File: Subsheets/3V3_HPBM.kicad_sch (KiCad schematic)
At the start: 7 parts

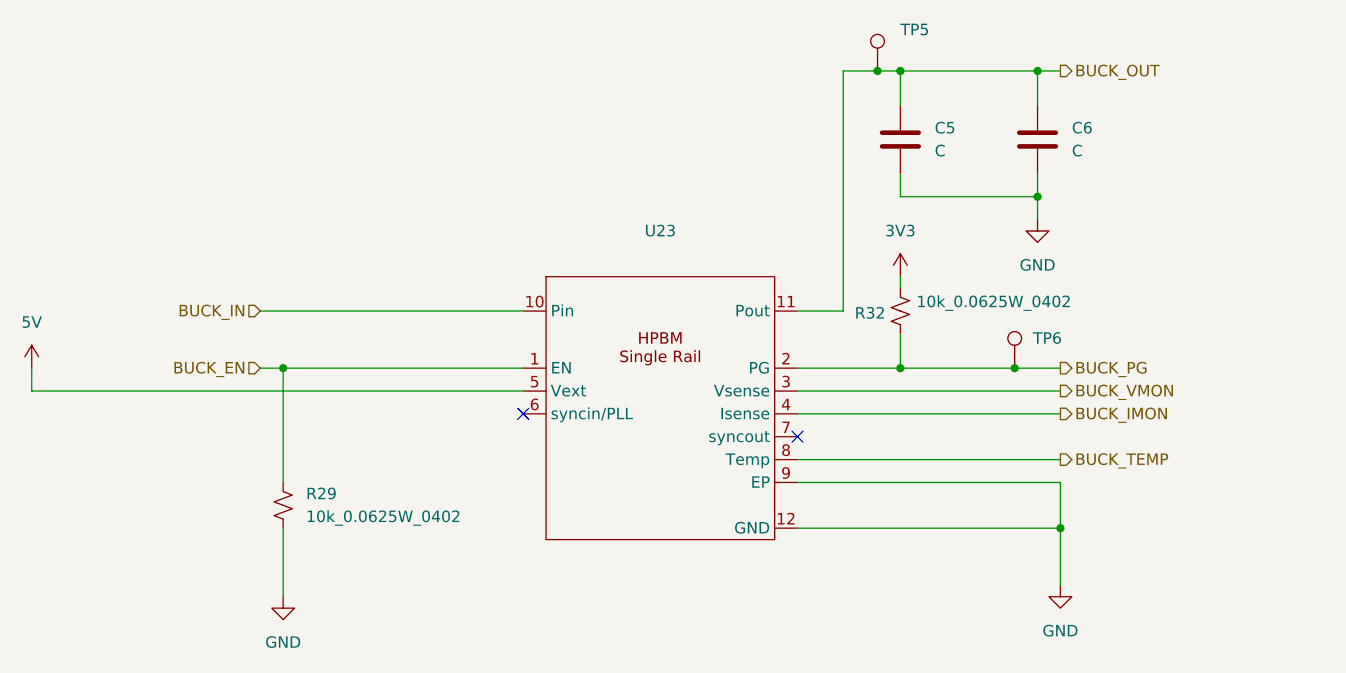
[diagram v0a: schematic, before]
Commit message: Schematic Update-1.1
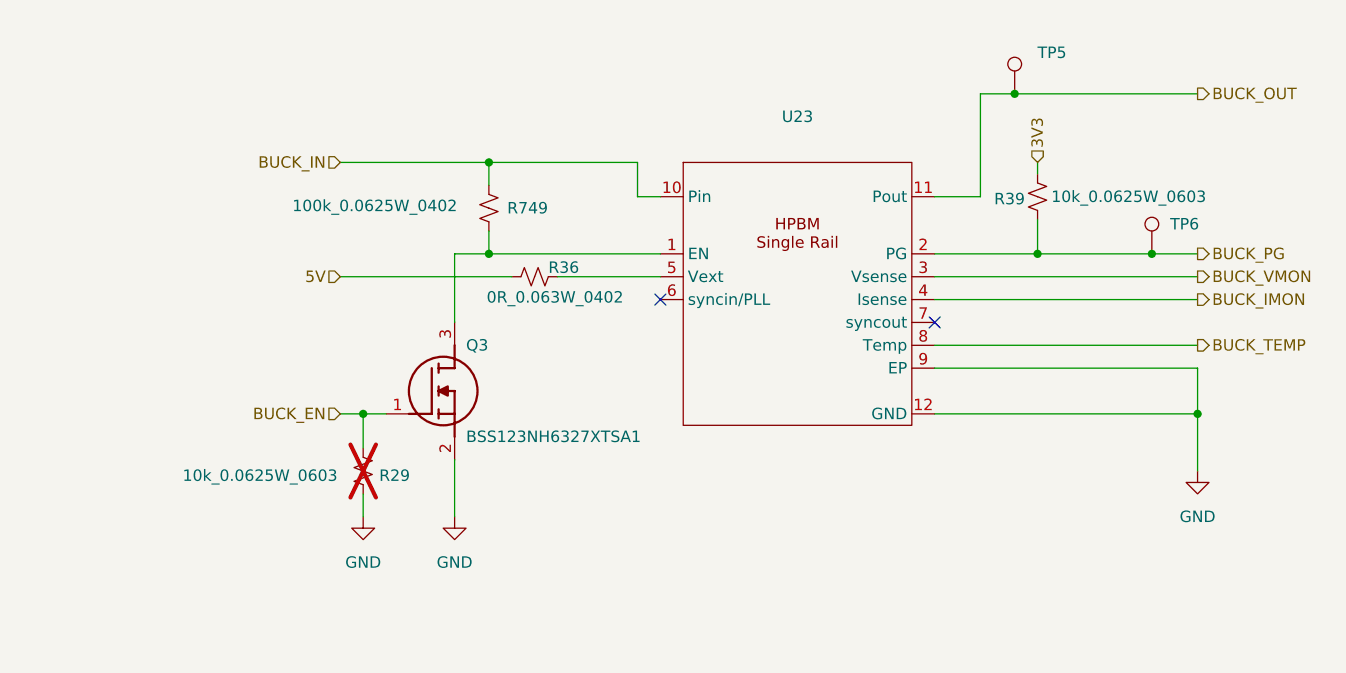
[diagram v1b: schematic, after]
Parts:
- removed C5, C6: C, symbol Device:C
- removed R32: 10k_0.0625W_0402, symbol Device:R_Small_US
- added Q3: BSS123NH6327XTSA1, SOT95P240X110-3N, symbol BSS123NH6327XTSA1:BSS123NH6327XTSA1
- added R36: 0R_0.063W_0402, Pixxel_Resistors:RES0402, symbol Device:R_Small_US
- added R39: 10k_0.0625W_0603, Pixxel_Resistors:RES0603, symbol Device:R_Small_US
- added R749: 100k_0.0625W_0402, Pixxel_Resistors:RES0402, symbol Device:R_Small_US
- R29: value 10k_0.0625W_0402 -> 10k_0.0625W_0603; footprint (none) -> Pixxel_Resistors:RES0603; Manufacturer Name (none) -> Vishay Dale; Manufacturer Part Number (none) -> TNPW060310K0BEEA; Price(INR) (none) -> 24.57; Temp_max (C) (none) -> 175; Temp_min (C) (none) -> -55; Vendor (none) -> Digikey; Vendor Part Number (none) -> TNP10.0KAATR-ND; now not fitted
- U23: value ~ -> (none)
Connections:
- net 3V3: now also R39.1
- net 5V: now also R36.2; no longer U23.5 (Vext)
- net BUCK_EN: now also Q3.1 (G); no longer U23.1 (EN)
- net BUCK_IN: now also R749.2
- net BUCK_PG: now also R39.2
- net GND: now also Q3.2 (S)
- new net: Q3.3 (D), R749.1, U23.1 (EN)
- new net: R36.1, U23.5 (Vext)
